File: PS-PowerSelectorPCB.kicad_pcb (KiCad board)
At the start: 2 copper layers, 47.6 x 44.2 mm, 27 parts, among them J1 SuppChargerIn, J2 PowerSupplyIn, J3 SuppChargerOut, J4 PowerSupplyOut, J5 Signals, J6 HV_Lockout, SW1 Power Source Selector

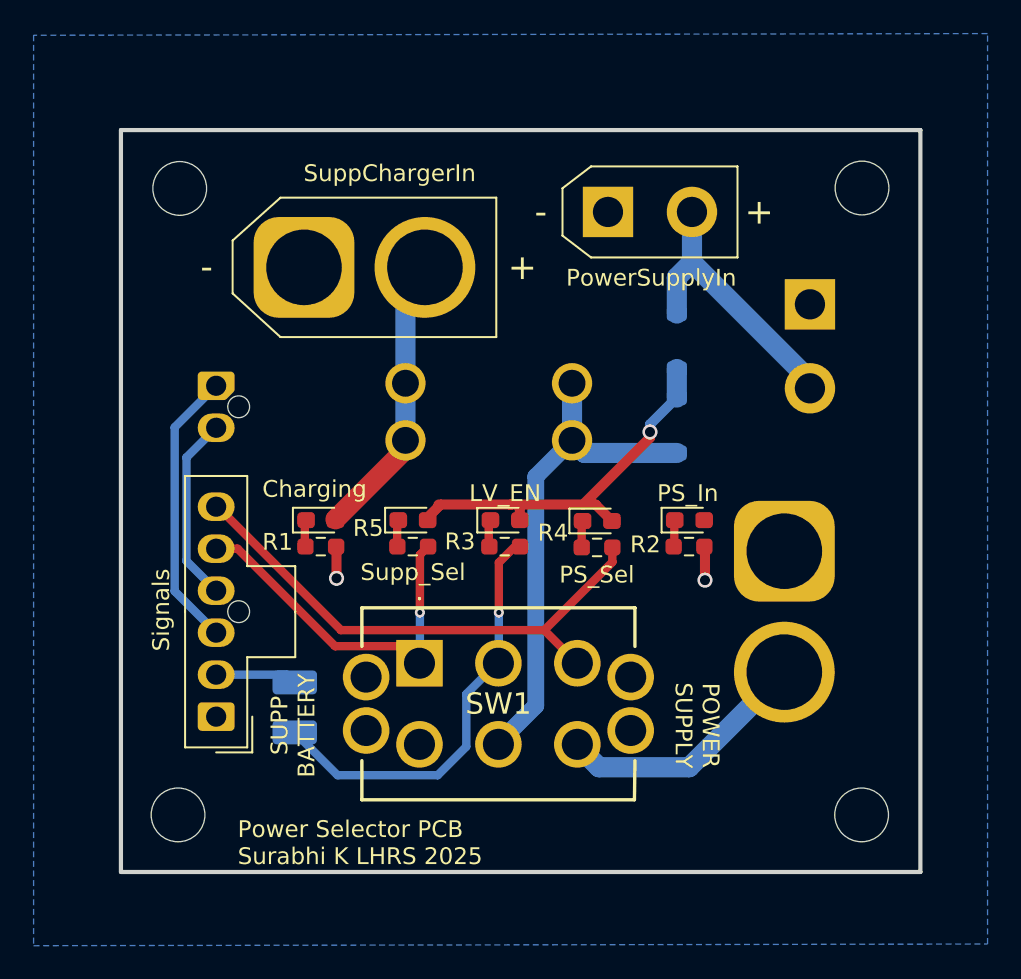
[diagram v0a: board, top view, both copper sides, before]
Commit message: silkscreens
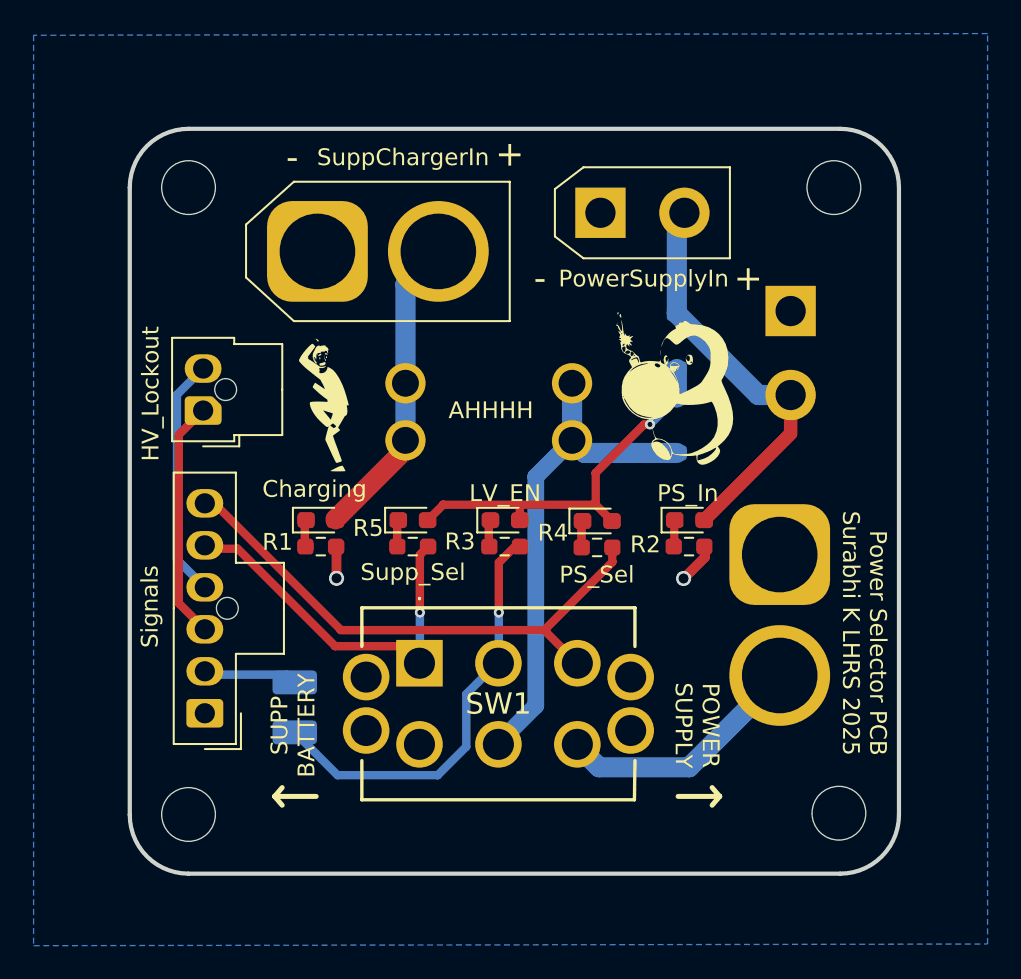
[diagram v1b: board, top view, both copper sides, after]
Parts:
- added G***: LOGO, LOGO, F.Cu at (106.0, 98.8)
- added G***: LOGO, LOGO, F.Cu at (85.5, 99.1)
- added G***: LOGO, LOGO, B.Cu at (78.0, 92.6)
- added G***: LOGO, LOGO, B.Cu at (86.4, 108.9)
- J6: moved to F.Cu
- moved H3 1.68 mm to (115.8, 86.2)
- moved J6 1.67 mm to (78.3, 99.5)
- moved LOGO1 1.63 mm to (105.8, 125.2)
- moved H2 1.35 mm to (116.2, 123.5)
- moved J1 1.24 mm to (85.1, 90.0)
- moved J4 1.22 mm to (113.3, 93.6)
- moved J5 0.70 mm to (78.4, 117.5)
- moved H4 0.63 mm to (77.4, 123.6)
- moved H1 0.53 mm to (77.4, 86.2)
- moved J2 0.45 mm to (102.0, 87.8)
- moved J3 0.34 mm to (112.6, 108.1)
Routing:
- net PS+: track 17.4 -> 24.6 mm
- net /HV_LO-: track 11.2 -> 14.4 mm
- net /HV_LO+: track 16.7 -> 14.3 mm
- net SuppChargerIn+: track 17.3 -> 18.5 mm
- net /LED+: track 23.5 -> 23.0 mm
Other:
- board size 47.6 x 44.2 mm -> 45.8 x 44.3 mm
- board text added: "AHHHH"
